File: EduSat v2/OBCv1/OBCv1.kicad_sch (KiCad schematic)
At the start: 36 parts, among them J1 Conn_02x20_Odd_Even, J2 USB_C_Receptacle_USB2.0_16P, J3 IDC Connector 2x10 20P, Q1 MMBT9014C, Q2 MMBT9014C, U1 ESP32-WROOM-32E, U2 CP2102N-Axx-xQFN28, U3 Ai-Thinker-Ra-02

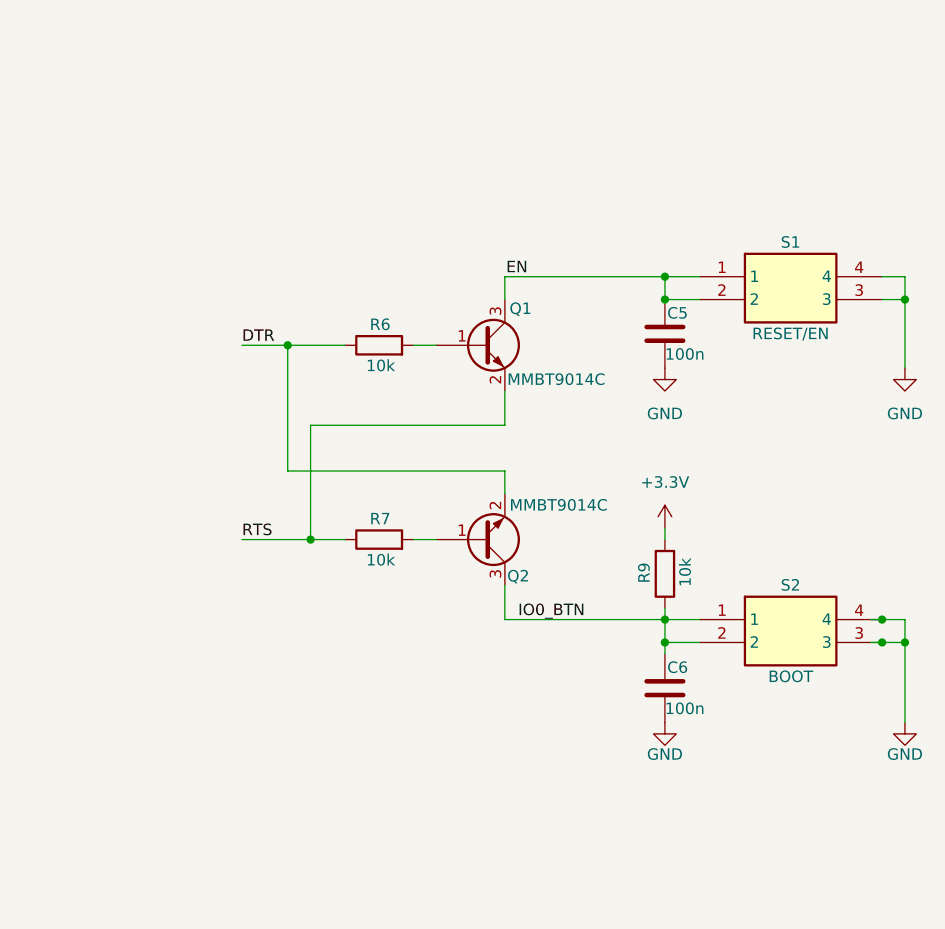
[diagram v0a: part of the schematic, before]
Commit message: Uploads
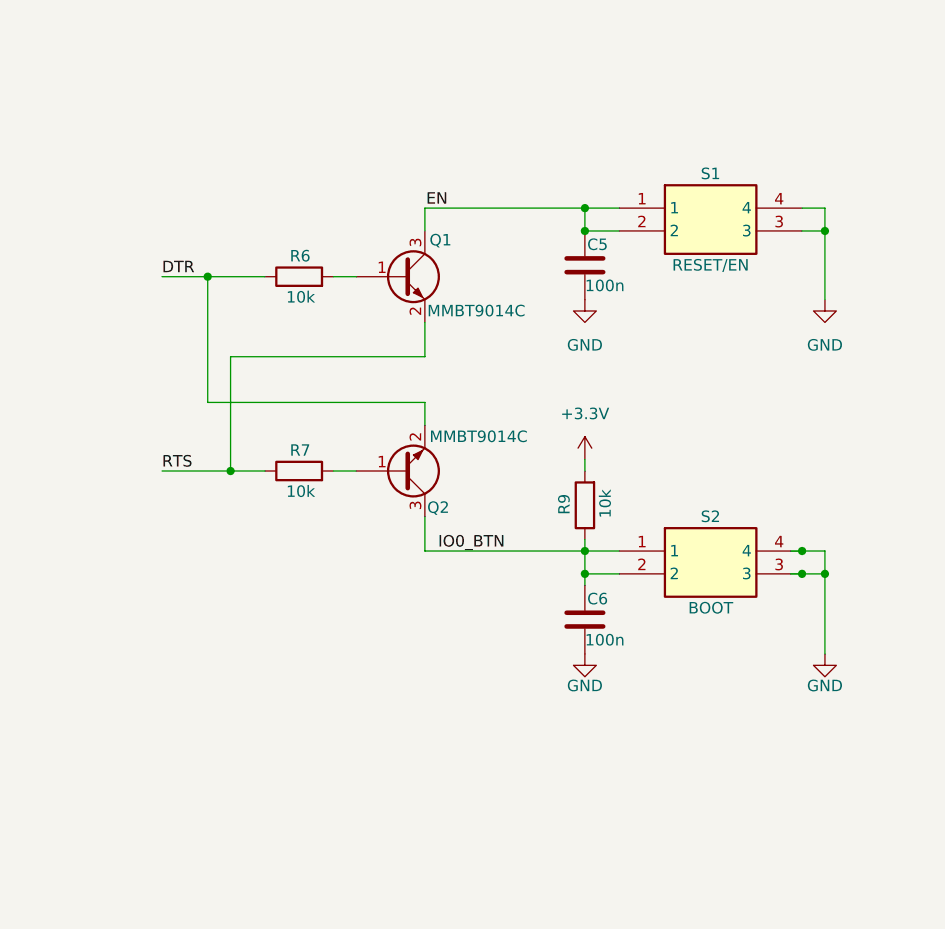
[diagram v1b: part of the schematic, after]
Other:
- moved on the sheet: C5, C6, Q1, Q2, R6, R7, R9, S1, S2
